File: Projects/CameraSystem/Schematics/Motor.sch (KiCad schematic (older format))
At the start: 2 parts, among them J13 Conn_02x02_Odd_Even, J14 Conn_02x05_Odd_Even

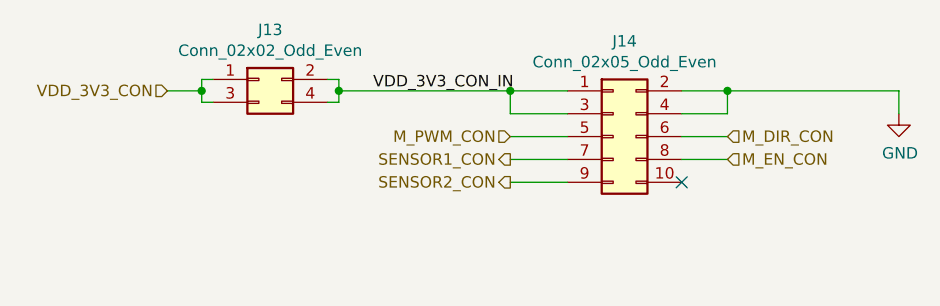
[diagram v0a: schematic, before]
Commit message: circuit updated
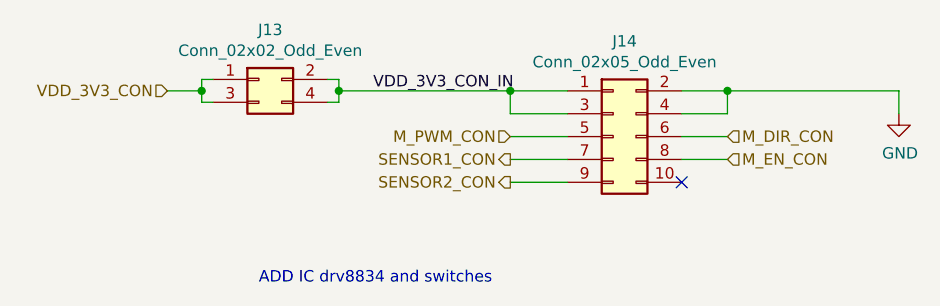
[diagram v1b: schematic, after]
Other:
- note added: "ADD IC drv8834 and switches"
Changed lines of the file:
@@
 	2100 1300 2150 1300
 Wire Wire Line
-	2150 1300 2150 1250
-Wire Wire Line
 	2150 1200 2100 1200
-Connection ~ 2150 1250
-Wire Wire Line
-	2150 1250 2150 1200
 Text Label 2300 1250 0    50   ~ 0
 VDD_3V3_CON_IN
@@
 Wire Wire Line
 	3150 1550 2900 1550
+Connection ~ 2150 1250
+Wire Wire Line
+	2150 1250 2150 1200
+Wire Wire Line
+	2150 1300 2150 1250
+Text Notes 1800 2100 0    50   ~ 0
+ADD IC drv8834 and switches
 $EndSCHEMATC
